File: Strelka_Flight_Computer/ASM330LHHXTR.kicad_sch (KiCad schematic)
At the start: 4 parts, among them U1 ASM330LHHXTR

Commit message: Changed design rules
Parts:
- C30: footprint Capacitor_SMD:C_0603_1608Metric -> Capacitor_SMD:C_0402_1005Metric
- U1: footprint QFN_LHHXTR_STM -> Footprints:QFN_LHHXTR_STM
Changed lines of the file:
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@@
       (effects (font (size 1.27 1.27)) (justify left))
     )
-    (property "Footprint" "Capacitor_SMD:C_0603_1608Metric" (at 190.754 115.062 0)
+    (property "Footprint" "Capacitor_SMD:C_0402_1005Metric" (at 190.754 115.062 0)
       (effects (font (size 1.27 1.27)) hide)
     )
@@
       (effects (font (size 1.27 1.27)) (justify left))
     )
-    (property "Footprint" "Capacitor_SMD:C_0603_1608Metric" (at 179.324 115.062 0)
+    (property "Footprint" "Capacitor_SMD:C_0402_1005Metric" (at 179.324 115.062 0)
       (effects (font (size 1.27 1.27)) hide)
     )
@@
       (effects (font (size 1.524 1.524)))
     )
-    (property "Footprint" "QFN_LHHXTR_STM" (at 127.508 86.868 0)
+    (property "Footprint" "Footprints:QFN_LHHXTR_STM" (at 127.508 86.868 0)
       (effects (font (size 1.27 1.27) italic) hide)
     )
-    (property "Datasheet" "ASM330LHHXTR" (at 127.508 86.868 0)
+    (property "Datasheet" "https://www.st.com/resource/en/datasheet/asm330lhhx.pdf" (at 127.508 86.868 0)
       (effects (font (size 1.27 1.27) italic) hide)
     )
@@
       (effects (font (size 1.27 1.27)) (justify left))
     )
-    (property "Footprint" "Capacitor_SMD:C_0603_1608Metric" (at 116.078 106.426 0)
+    (property "Footprint" "Capacitor_SMD:C_0402_1005Metric" (at 116.078 106.426 0)
       (effects (font (size 1.27 1.27)) hide)
     )

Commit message: Routing starting
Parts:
- C30: LCSC (none) -> C15525
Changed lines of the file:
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@@
+      (effects (font (size 1.27 1.27)) hide)
+    )
+    (property "LCSC" "C15525" (at 190.754 115.062 0)
       (effects (font (size 1.27 1.27)) hide)
     )

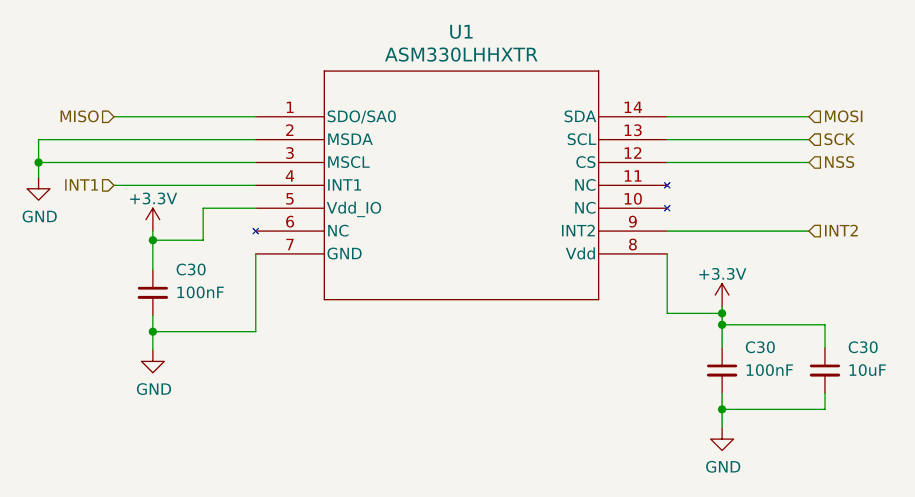
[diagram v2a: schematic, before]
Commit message: Continued routing
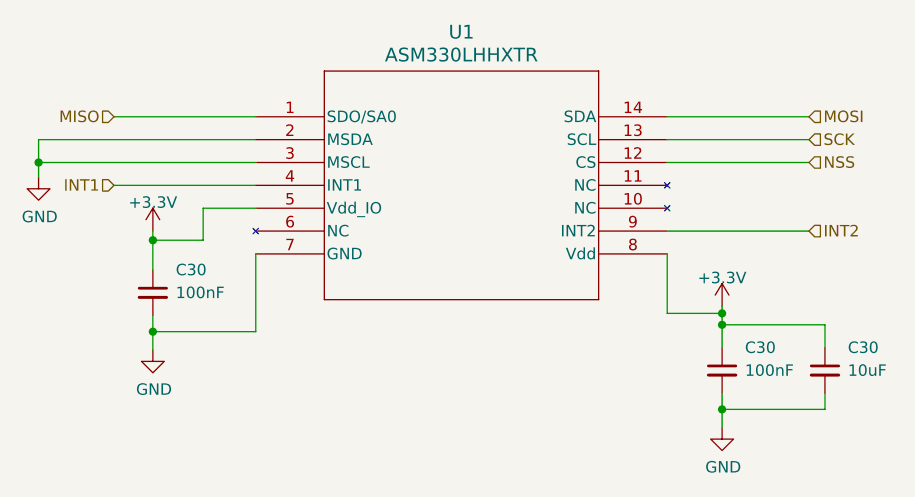
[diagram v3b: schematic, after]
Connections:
- net +3V3 renamed +3.3V
